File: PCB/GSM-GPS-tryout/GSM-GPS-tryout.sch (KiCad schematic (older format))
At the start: 0 parts

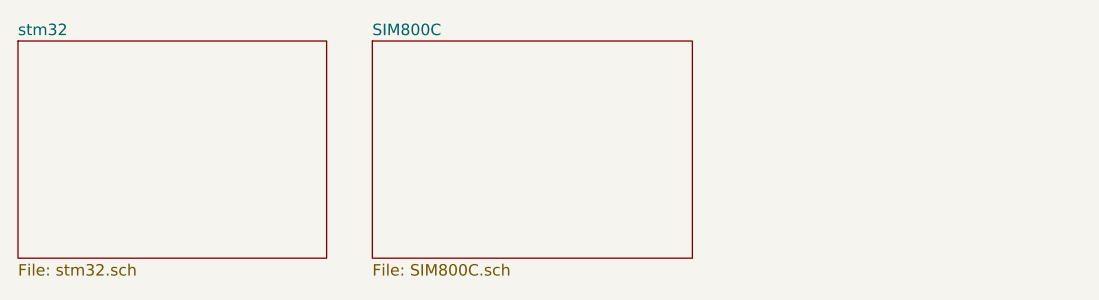
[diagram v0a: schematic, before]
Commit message: update,
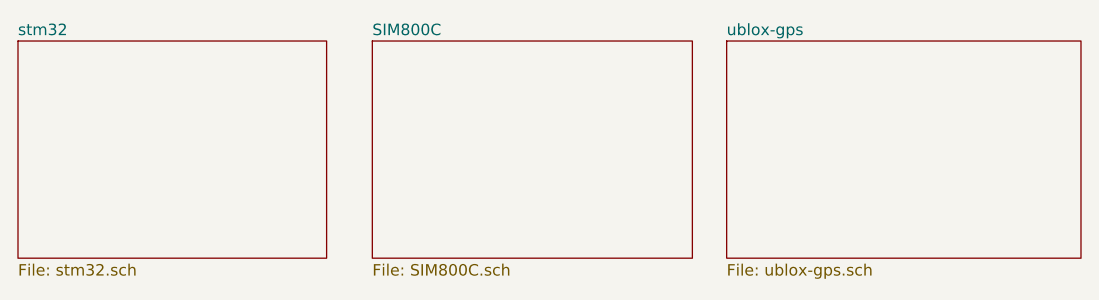
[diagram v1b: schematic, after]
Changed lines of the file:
@@
 $Descr A3 16535 11693
 encoding utf-8
-Sheet 1 3
+Sheet 1 4
 Title ""
 Date ""
@@
 F1 "SIM800C.sch" 50
 $EndSheet
+$Sheet
+S 4250 850  1550 950
+U 5BBADC15
+F0 "ublox-gps" 50
+F1 "ublox-gps.sch" 50
+$EndSheet
 $EndSCHEMATC
